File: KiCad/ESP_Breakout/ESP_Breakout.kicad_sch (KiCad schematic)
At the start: 19 parts, among them J1 Conn_01x15_Socket, J2 Conn_01x15_Socket, J3 Conn_01x03_Pin, J4 Conn_01x03_Pin, J5 Conn_01x03_Pin, J6 Conn_01x03_Pin

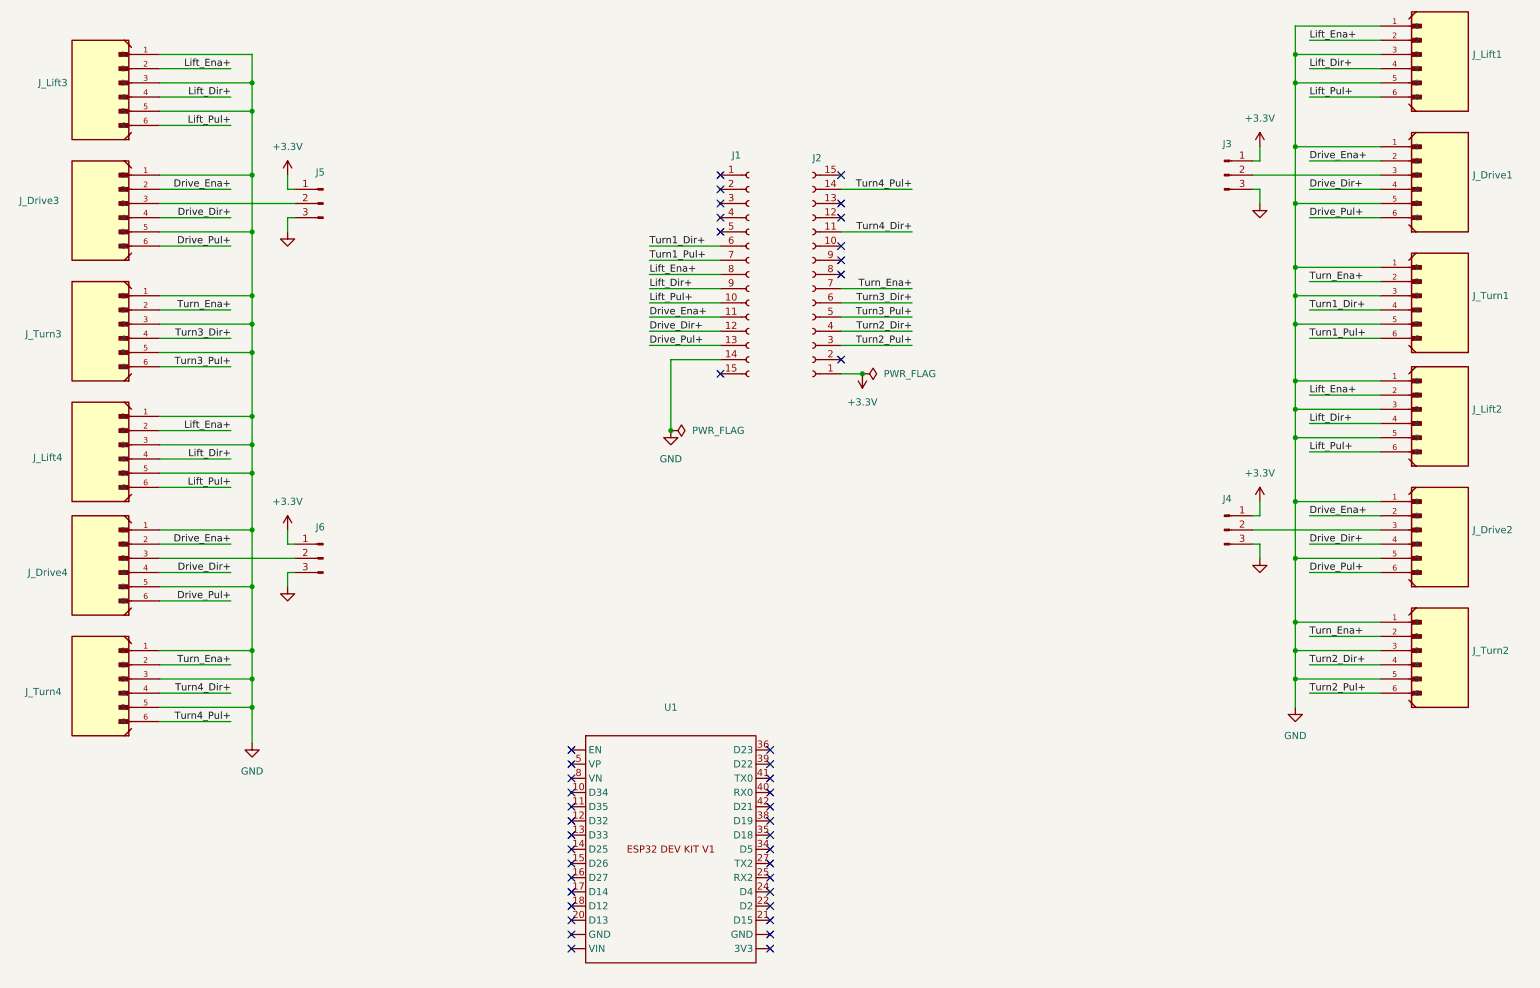
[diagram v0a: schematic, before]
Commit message: starting pcb layout
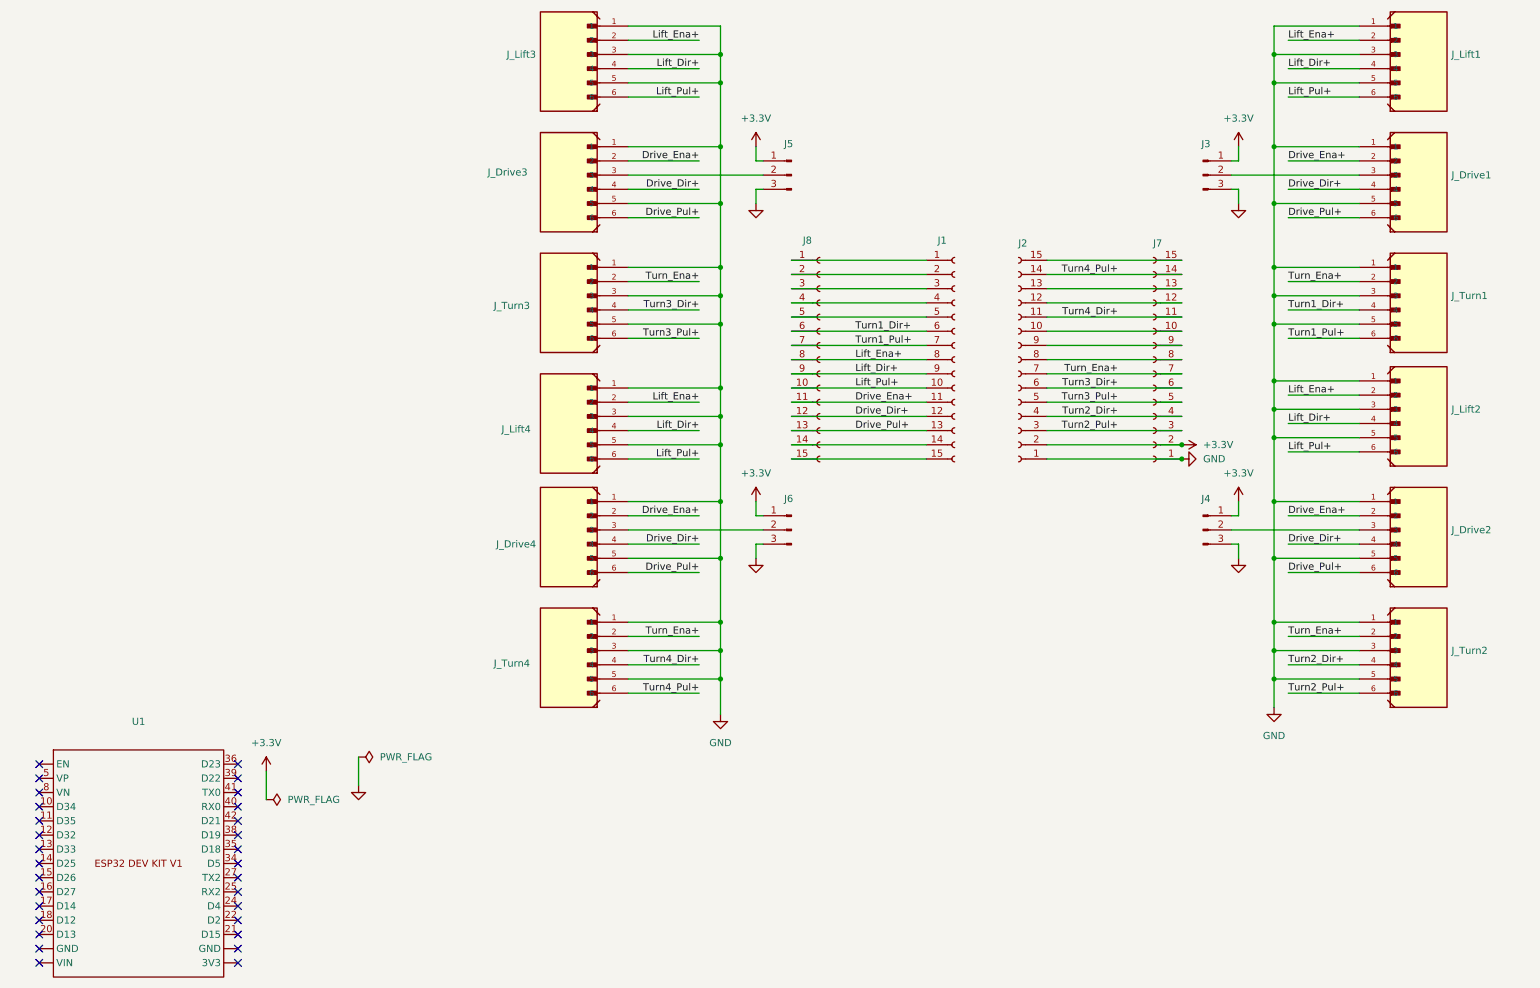
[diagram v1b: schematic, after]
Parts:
- added J7, J8: Conn_01x15_Socket, Connector_PinSocket_2.54mm:PinSocket_1x15_P2.54mm_Vertical, symbol Connector:Conn_01x15_Socket
- J3, J4, J5, J6: footprint Connector_PinHeader_1.00mm:PinHeader_1x03_P1.00mm_Vertical -> Connector_PinHeader_2.54mm:PinHeader_1x03_P2.54mm_Vertical
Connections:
- net +3.3V: now also J2.2 (Pin_2), J7.2 (Pin_2); no longer J2.1 (Pin_1)
- net Drive_Dir+: now also J8.12 (Pin_12)
- net Drive_Ena+: now also J8.11 (Pin_11)
- net Drive_Pul+: now also J8.13 (Pin_13)
- net GND: now also J2.1 (Pin_1), J7.1 (Pin_1); no longer J1.14 (Pin_14)
- net Lift_Dir+: now also J8.9 (Pin_9)
- net Lift_Ena+: now also J8.8 (Pin_8)
- net Lift_Pul+: now also J8.10 (Pin_10)
- net Turn1_Dir+: now also J8.6 (Pin_6)
- net Turn1_Pul+: now also J8.7 (Pin_7)
- net Turn2_Dir+: now also J7.4 (Pin_4)
- net Turn2_Pul+: now also J7.3 (Pin_3)
- net Turn3_Dir+: now also J7.6 (Pin_6)
- net Turn3_Pul+: now also J7.5 (Pin_5)
- net Turn4_Dir+: now also J7.11 (Pin_11)
- net Turn4_Pul+: now also J7.14 (Pin_14)
- net Turn_Ena+: now also J7.7 (Pin_7)
- net at J1.1 (Pin_1): now also J8.1 (Pin_1)
- net at J1.15 (Pin_15): now also J8.15 (Pin_15)
- net at J1.2 (Pin_2): now also J8.2 (Pin_2)
- net at J1.3 (Pin_3): now also J8.3 (Pin_3)
- net at J1.4 (Pin_4): now also J8.4 (Pin_4)
- net at J1.5 (Pin_5): now also J8.5 (Pin_5)
- net at J2.10 (Pin_10): now also J7.10 (Pin_10)
- net at J2.12 (Pin_12): now also J7.12 (Pin_12)
- net at J2.13 (Pin_13): now also J7.13 (Pin_13)
- net at J2.15 (Pin_15): now also J7.15 (Pin_15)
- net at J2.8 (Pin_8): now also J7.8 (Pin_8)
- net at J2.9 (Pin_9): now also J7.9 (Pin_9)
- new net: J1.14 (Pin_14), J8.14 (Pin_14)
- no-connect marks 43 -> 30
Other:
- moved on the sheet: J1, J2, J3, J4, J5, J6, J_Drive1, J_Drive2, J_Drive3, J_Drive4, J_Lift1, J_Lift2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
